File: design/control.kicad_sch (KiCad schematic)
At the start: 20 parts, among them J3 Conn-OScope, J3 SMB, J4 Conn-OScope, J4 SMA, J5 USB_C_Receptacle_USB2.0_14P, U1 STM32F303RETx, U4 CP2102N-Axx-xQFN20

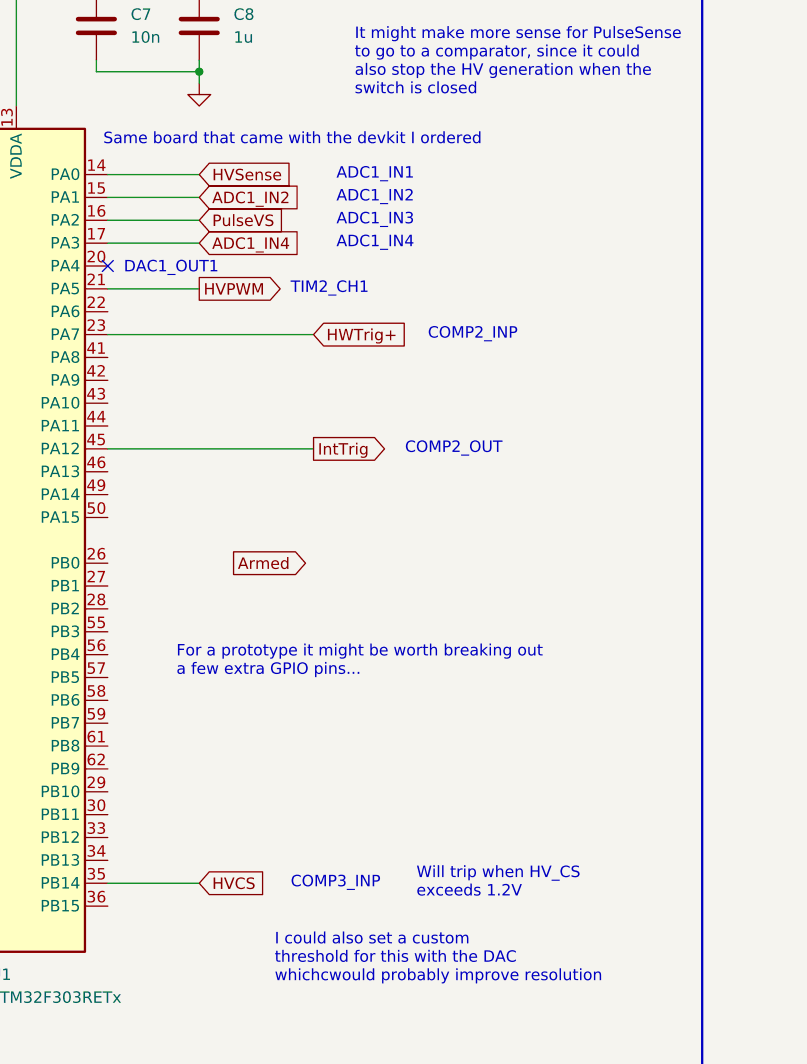
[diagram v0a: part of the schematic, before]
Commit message: _
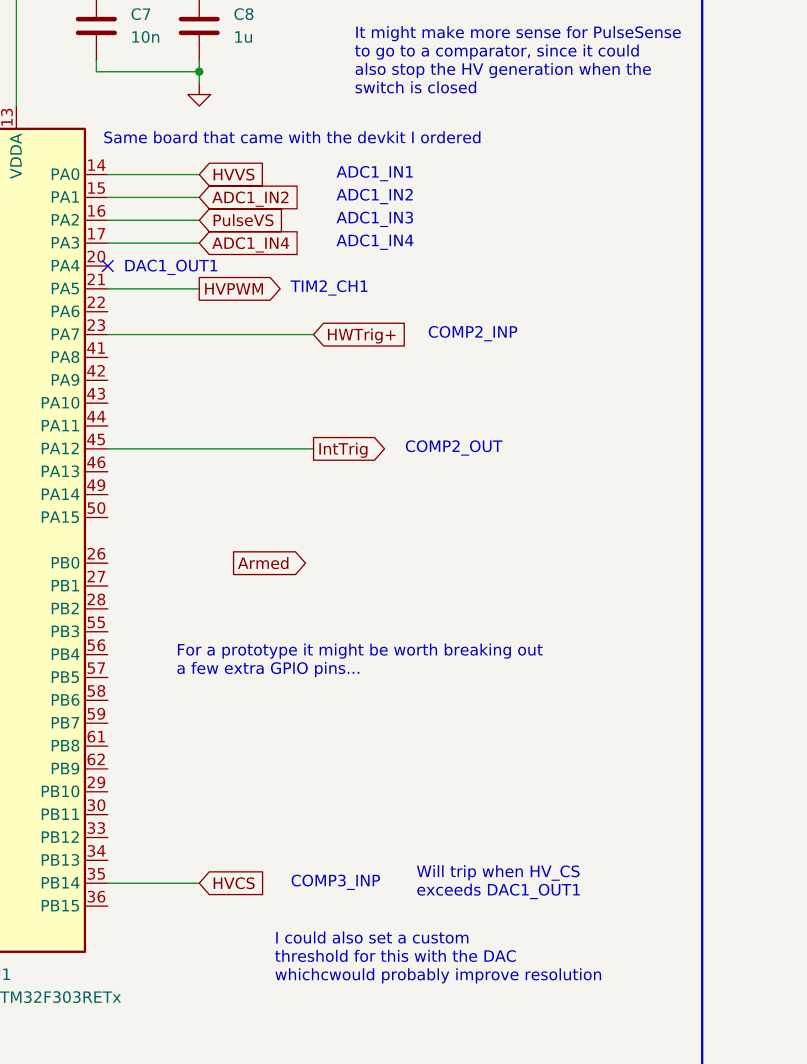
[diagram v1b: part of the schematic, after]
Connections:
- net HVSense renamed HVVS
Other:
- note added: "Will trip when HV_CS exceeds DAC1_OUT1"
- note removed: "Will trip when HV_CS exceeds 1.2V"
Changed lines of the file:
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@@
 		)
 	)
-	(text "Will trip when HV_CS\nexceeds 1.2V"
+	(text "Will trip when HV_CS\nexceeds DAC1_OUT1"
 		(exclude_from_sim no)
 		(at 248.92 128.27 0)
@@
 		)
 	)
-	(global_label "HVSense"
+	(global_label "HVVS"
 		(shape input)
 		(at 224.79 49.53 0)
@@
 		)
 		(property "Intersheetrefs" "${INTERSHEET_REFS}"
-			(at 235.7581 49.53 0)
+			(at 232.4924 49.53 0)
 			(effects
 				(font
